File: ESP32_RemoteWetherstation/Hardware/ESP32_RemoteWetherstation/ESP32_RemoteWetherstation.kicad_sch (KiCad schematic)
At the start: 5 parts, among them J301 BOOT, J302 UART, U303 ESP32-S3-MINI-1

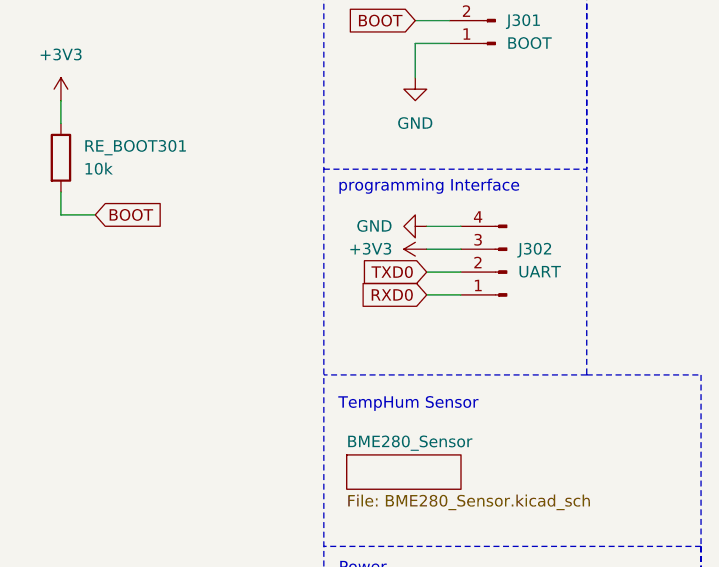
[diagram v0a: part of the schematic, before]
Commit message: stitching/PowerModule
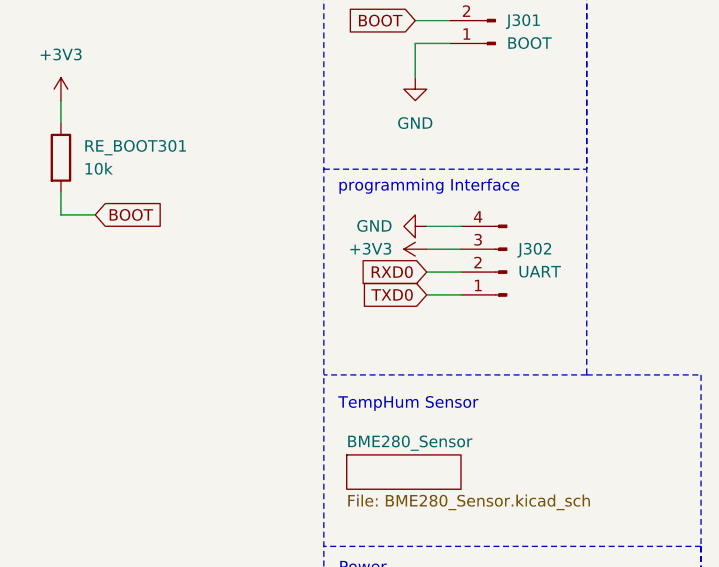
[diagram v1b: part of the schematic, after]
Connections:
- net RXD0: now also J302.2 (Pin_2); no longer J302.1 (Pin_1)
- net TXD0: now also J302.1 (Pin_1); no longer J302.2 (Pin_2)
